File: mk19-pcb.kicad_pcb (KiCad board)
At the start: 2 copper layers, 130 x 85 mm, 90 parts, among them J1 Conn_01x02_Socket, J10 Conn_01x02_Socket, J11 Conn_01x02_Socket, J2 Conn_01x02_Socket, J4 Conn_01x02_Socket, J7 Conn_01x02_Socket, J9 Conn_01x02_Socket, T1 Conn_01x01_Socket, T10 Conn_01x01_Socket, U1 AZC199-04S-MS, U10 8_01A0_008200, U11 8_01A0_008200, U2 1N4148W_C81598, U3 1N4148W_C81598, U4 1N4148W_C81598, U5 1N4148W_C81598, U6 1N4148W_C81598, U9 8_01A0_008200

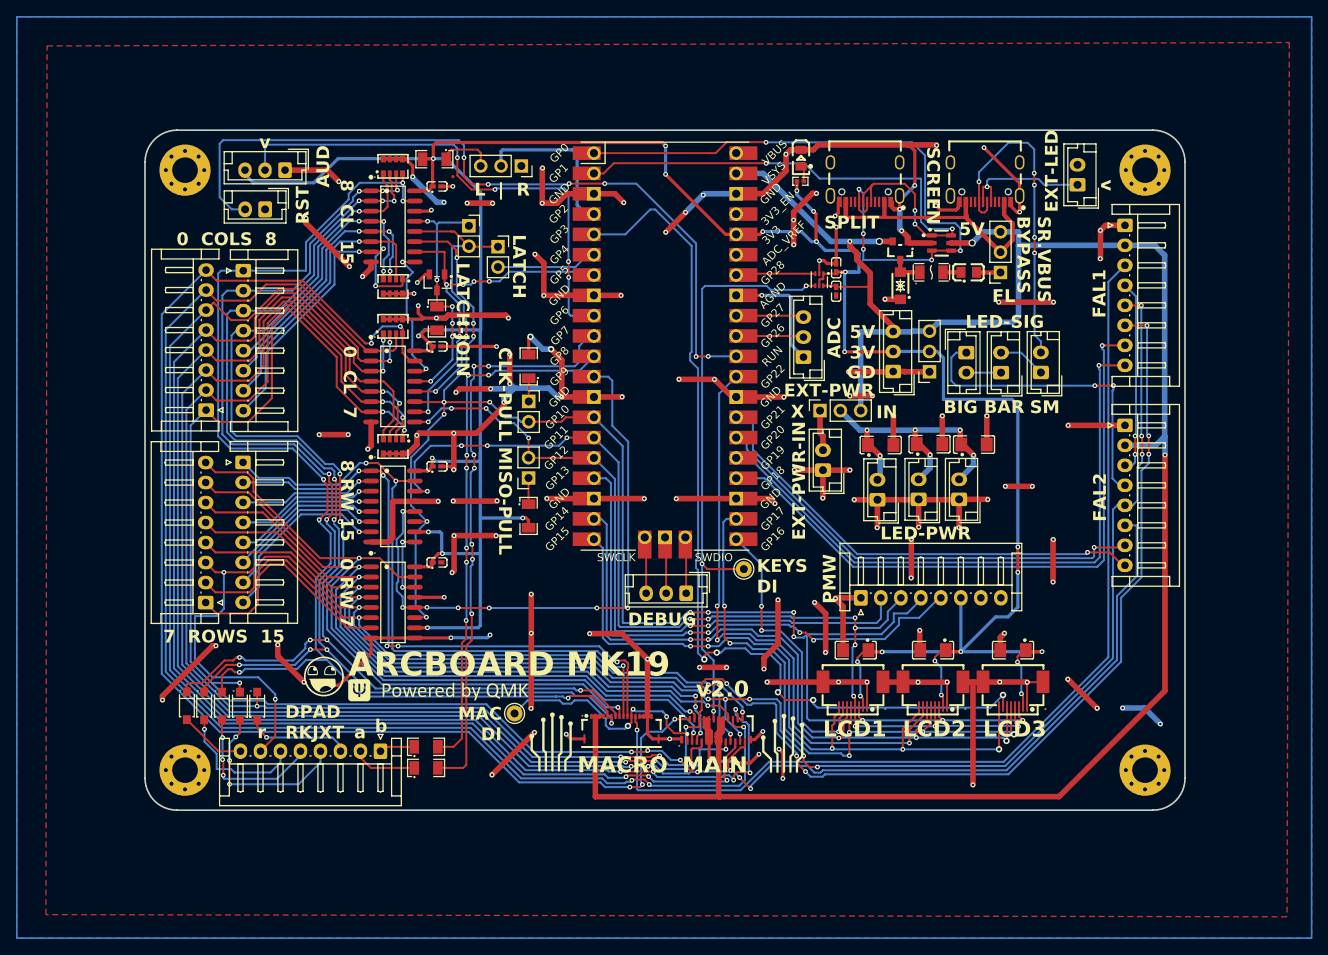
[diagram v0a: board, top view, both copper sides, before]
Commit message: production files
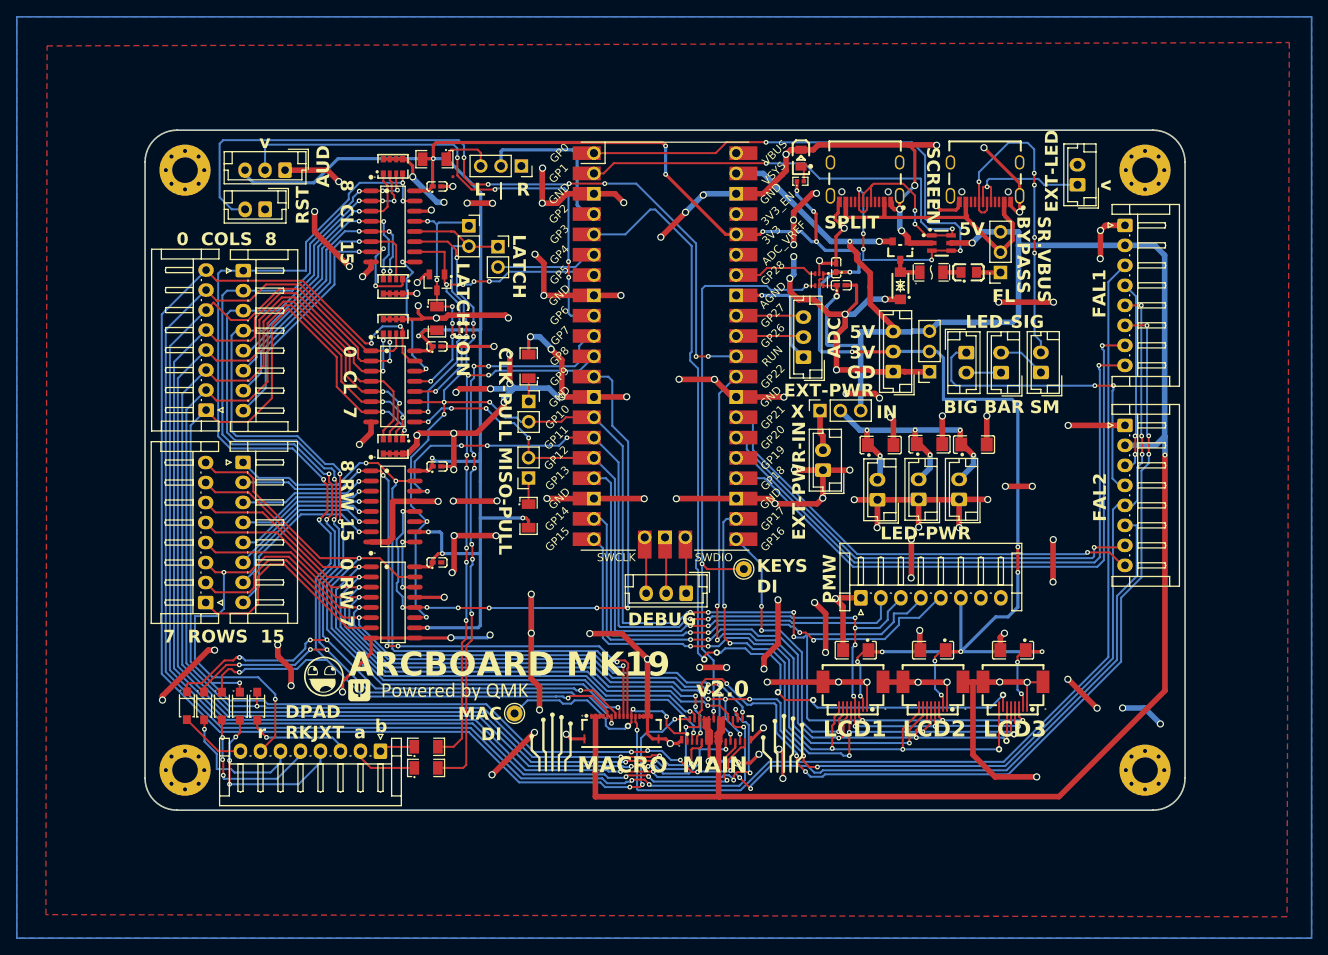
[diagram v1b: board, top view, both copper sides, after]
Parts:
- moved C6 0.99 mm to (167.0, 69.4), turned to 0 degrees
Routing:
- net GND: track 641.5 -> 688.5 mm
- net VCC: track 276.7 -> 284.7 mm, vias 4 -> 5
- net +3V3: track 362.3 -> 366.8 mm
- net LED_DI_3v3: track 9.96 -> 10.6 mm
